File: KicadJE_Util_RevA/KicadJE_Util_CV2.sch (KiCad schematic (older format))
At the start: 53 parts, among them J201 SawOut3, J202 SineOut4, Q201 MMBT3906, Q202 UMX1N, SW201 Octave (3 state), U201 TL072, U202 TL072

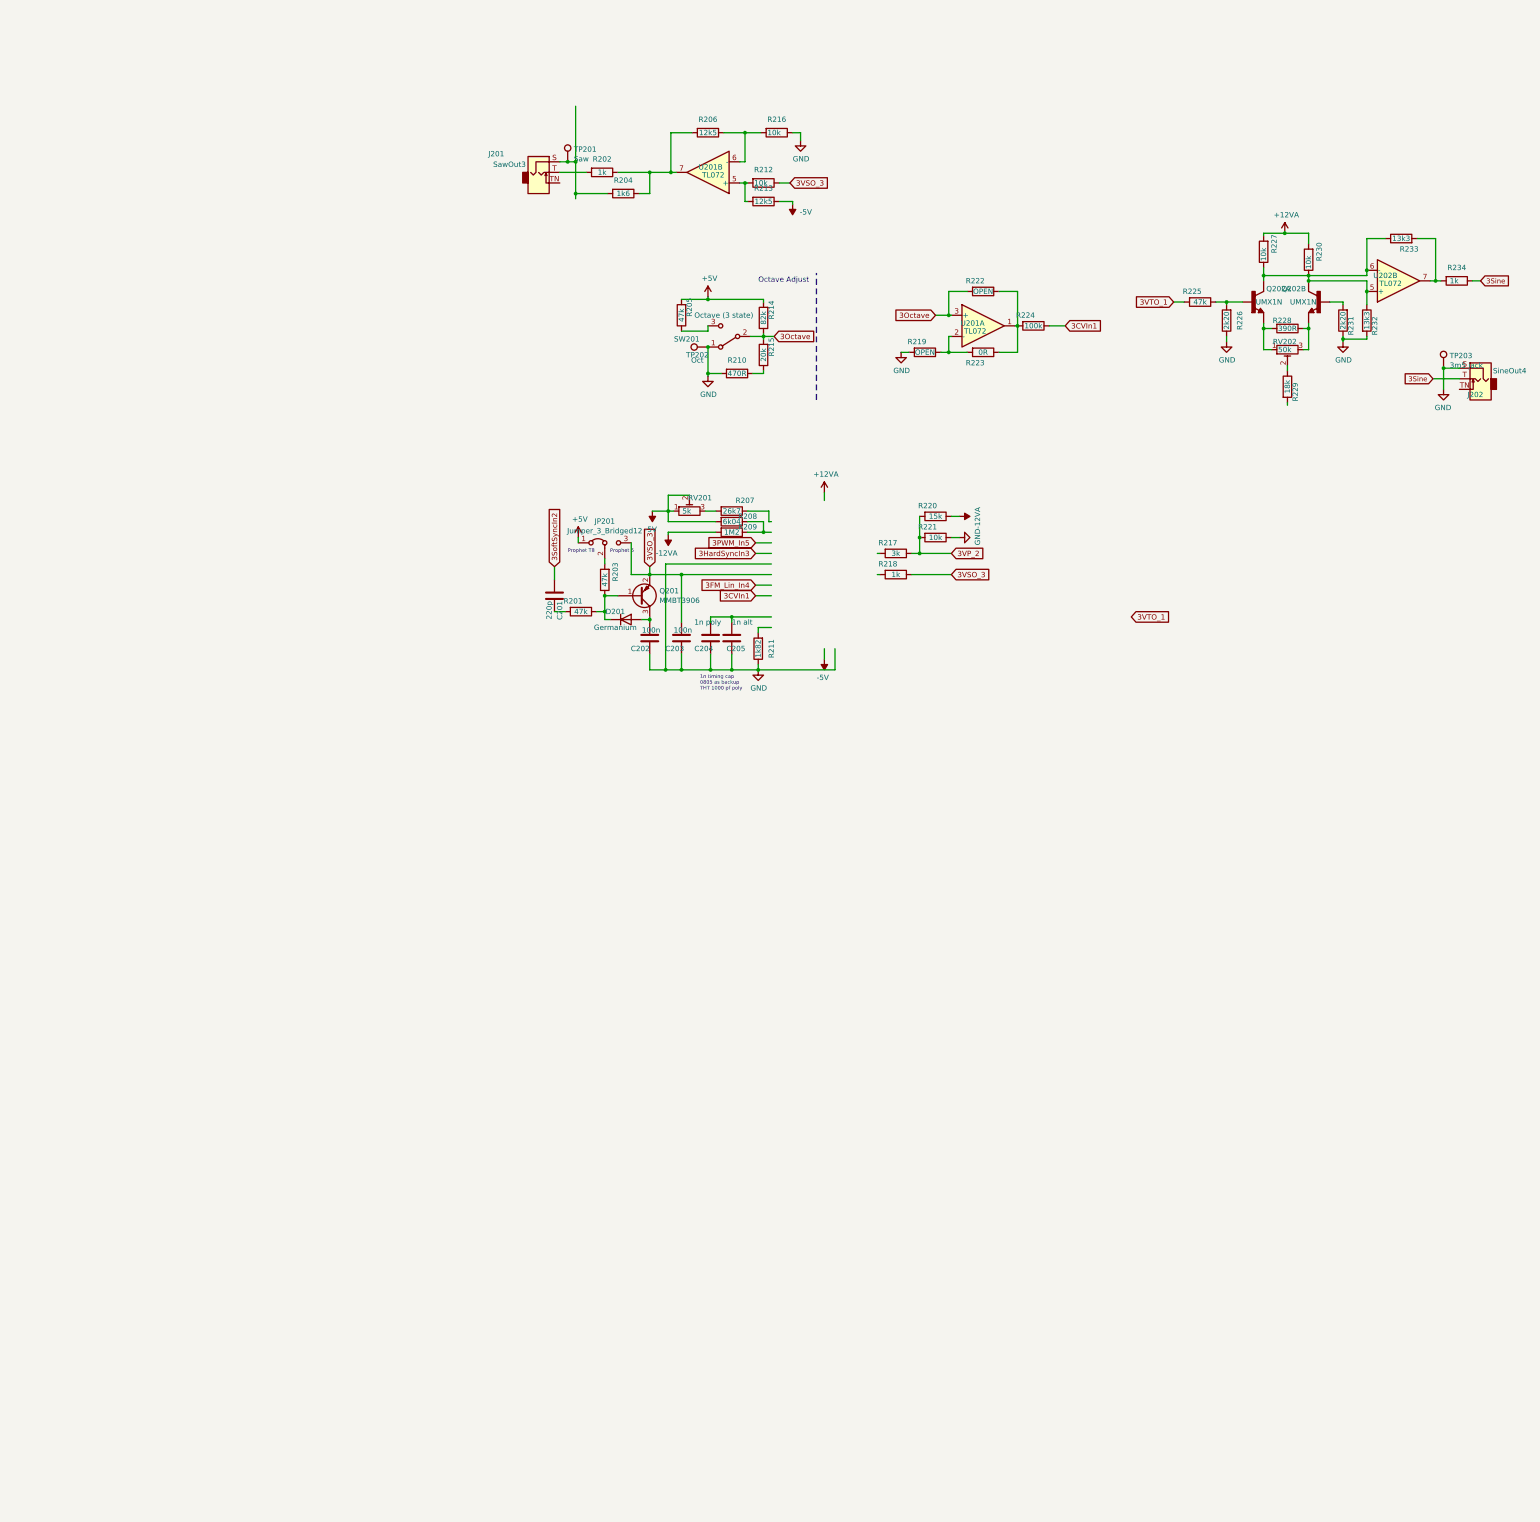
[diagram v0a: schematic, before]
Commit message: fix flow
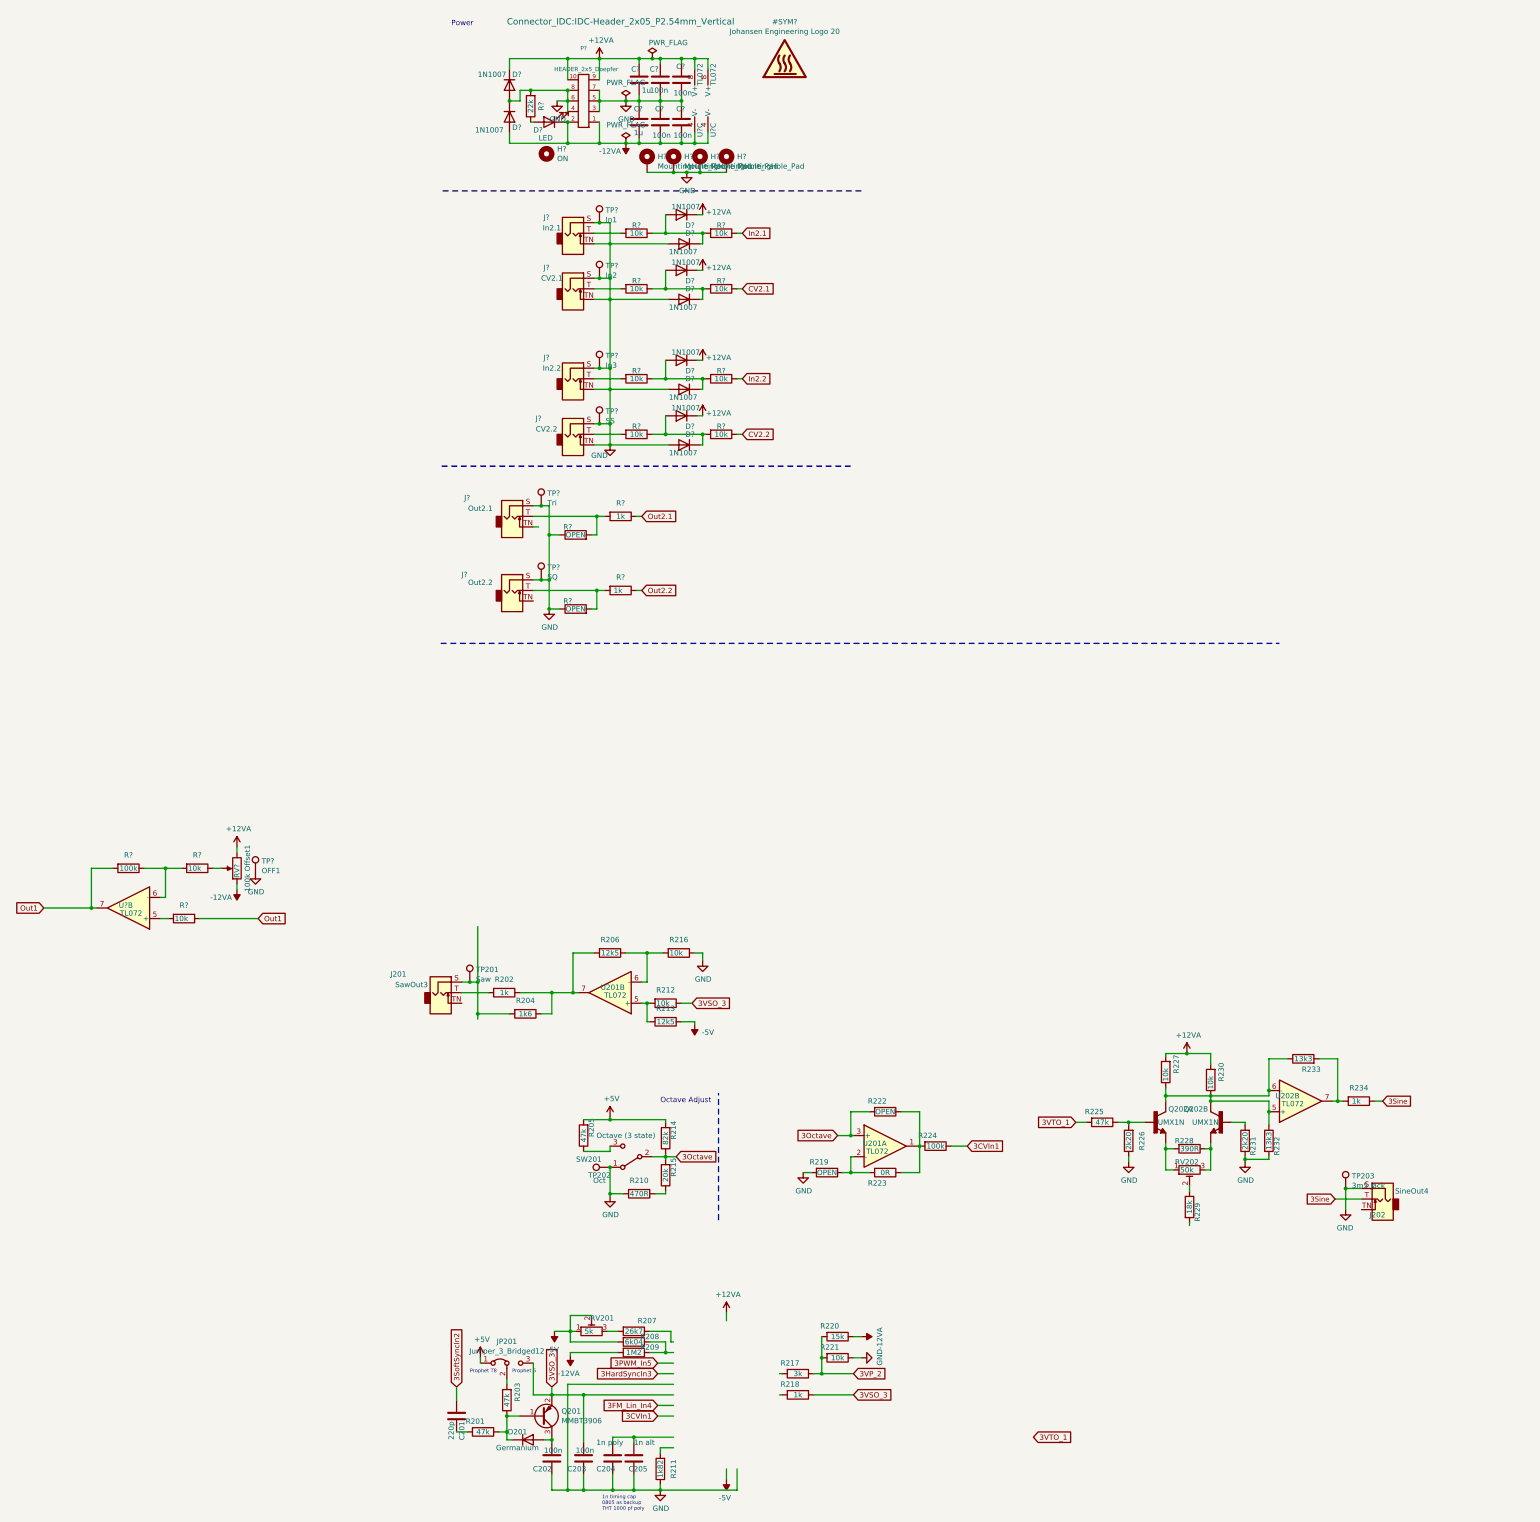
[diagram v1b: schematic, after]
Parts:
- added C? (x2): 1u, Capacitor_SMD:C_1206_3216Metric_Pad1.42x1.75mm_HandSolder, symbol Device:C
- added C? (x4): 100n, Capacitor_SMD:C_0805_2012Metric_Pad1.15x1.40mm_HandSolder, symbol Device:C
- added D? (x10): 1N1007, Diode_SMD:D_SOD-123, symbol Device:D
- added D?: LED, LED_SMD:LED_0805_2012Metric_Pad1.15x1.40mm_HandSolder, symbol Device:LED
- added H? (x4): MountingHole_Pad, AJ:MountingHole_Eurorack3, symbol Mechanical:MountingHole_Pad
- added H?: ON, AJ:LED_Hole_3mm, symbol Mechanical:MountingHole
- added J?: In2.1, AJ-Dropbox-Kicad:PJ301SM, symbol Connector:AudioJack2_SwitchT
- added J?: CV2.1, AJ-Dropbox-Kicad:PJ301SM, symbol Connector:AudioJack2_SwitchT
- added J?: Out2.1, AJ-Dropbox-Kicad:PJ301SM, symbol Connector:AudioJack2_SwitchT
- added J?: CV2.2, AJ-Dropbox-Kicad:PJ301SM, symbol Connector:AudioJack2_SwitchT
- added J?: Out2.2, AJ-Dropbox-Kicad:PJ301SM, symbol Connector:AudioJack2_SwitchT
- added J?: In2.2, AJ-Dropbox-Kicad:PJ301SM, symbol Connector:AudioJack2_SwitchT
- added P?: HEADER_2x5_Doepfer, Connector_IDC:IDC-Header_2x05_P2.54mm_Vertical, symbol Eurorack:HEADER_2x5_Doepfer
- added R? (x10): 10k, Resistor_SMD:R_0805_2012Metric_Pad1.15x1.40mm_HandSolder, symbol Device:R
- added R? (x2): 1k, Resistor_SMD:R_0805_2012Metric_Pad1.15x1.40mm_HandSolder, symbol Device:R
- added R?: 22k, Resistor_SMD:R_0805_2012Metric_Pad1.15x1.40mm_HandSolder, symbol Device:R
- added R? (x2): OPEN, Resistor_SMD:R_0805_2012Metric_Pad1.15x1.40mm_HandSolder, symbol Device:R
- added R?: 100k, Resistor_SMD:R_0805_2012Metric_Pad1.15x1.40mm_HandSolder, symbol Device:R
- added RV?: 100k Offset1, AJ-Dropbox-Kicad:Potentiometer_China_RK09_Single_Vertical_AJ, symbol Envelope-cache-2018-08-04-13-00-04:POT
- added TP?: Tri, AJ:Jack_6m3, symbol Connector:TestPoint
- added TP?: SQ, AJ:Jack_6m3, symbol Connector:TestPoint
- added TP?: SS, AJ:Jack_6m3, symbol Connector:TestPoint
- added TP?: In3, AJ:Jack_6m3, symbol Connector:TestPoint
- added TP?: In2, AJ:Jack_6m3, symbol Connector:TestPoint
- added TP?: In1, AJ:Jack_6m3, symbol Connector:TestPoint
- added TP?: OFF1, AJ:Pot_6m3_scale1, symbol Connector:TestPoint
- added U? (x3): TL072, AJ-Dropbox-Kicad:AJ_SO-8_5.3x6.2mm_P1.27mm, symbol Amplifier_Operational:TL072
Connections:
- net labels added: CV2.1, CV2.2, In2.1, In2.2, Out1, Out2.1, Out2.2
- wire segments 170 -> 319
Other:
- note added: "Power"
- moved on the sheet: C201, C202, C203, C204, C205, D201, J201, J202, JP201, Q201, Q202A, Q202B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

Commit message: Glide initiated
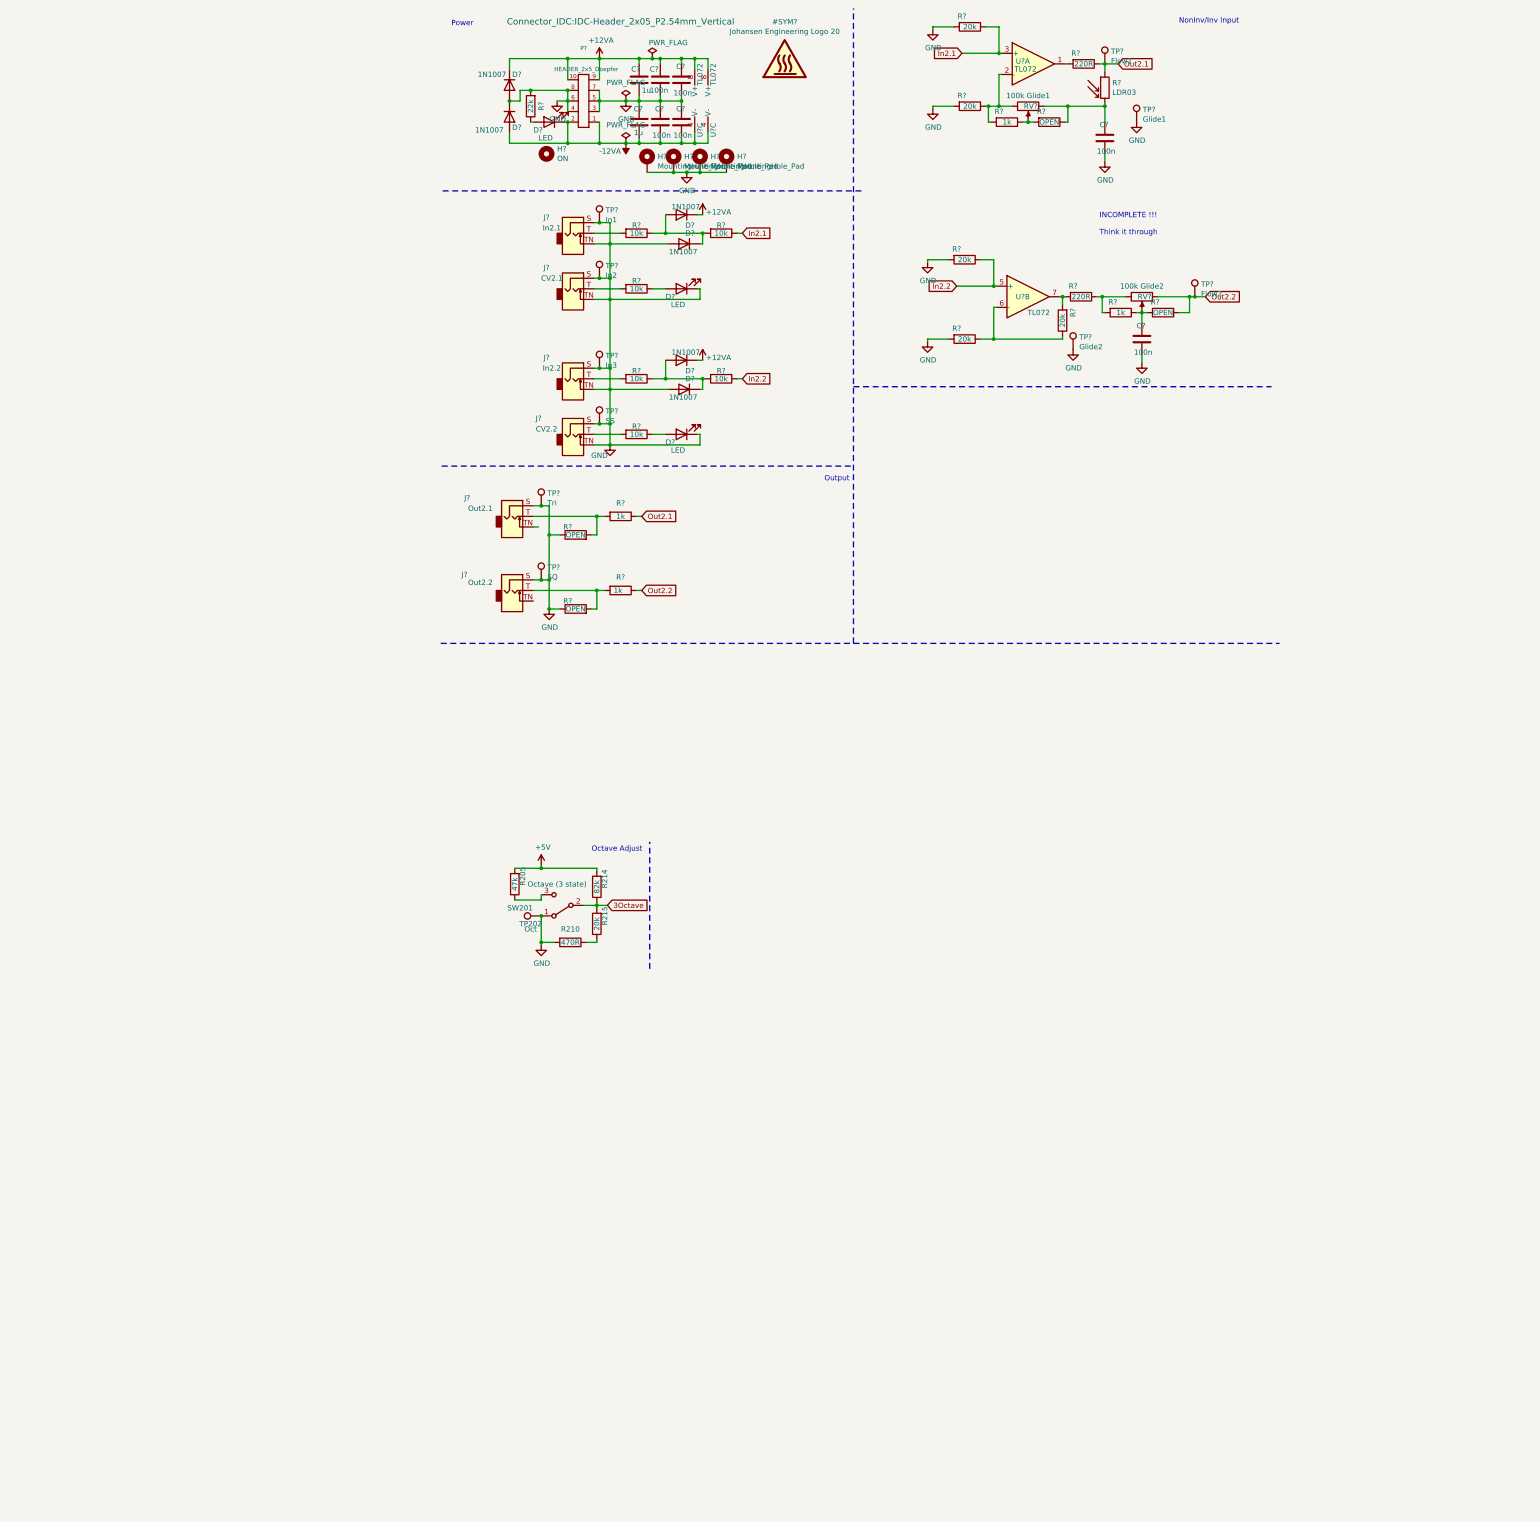
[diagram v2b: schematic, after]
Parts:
- removed C201: 220p, Capacitor_SMD:C_0805_2012Metric_Pad1.15x1.40mm_HandSolder, symbol Device:C
- removed C202, C203: 100n, Capacitor_SMD:C_0805_2012Metric_Pad1.15x1.40mm_HandSolder, symbol Device:C
- removed C204: 1n poly, Capacitor_THT:C_Rect_L7.0mm_W2.0mm_P5.00mm, symbol Device:C
- removed C205: 1n alt, Capacitor_SMD:C_0805_2012Metric_Pad1.15x1.40mm_HandSolder, symbol Device:C
- removed D201: Germanium, Diode_THT:D_A-405_P7.62mm_Horizontal, symbol Device:D
- removed D? (x4): 1N1007, Diode_SMD:D_SOD-123, symbol Device:D
- removed J201: SawOut3, AJ-Dropbox-Kicad:PJ301SM, symbol Connector:AudioJack2_SwitchT
- removed J202: SineOut4, AJ-Dropbox-Kicad:PJ301SM, symbol Connector:AudioJack2_SwitchT
- removed JP201: Jumper_3_Bridged12, Jumper:SolderJumper-3_P1.3mm_Bridged12_Pad1.0x1.5mm_NumberLabels, symbol Jumper:Jumper_3_Bridged12
- removed Q201: MMBT3906, Package_TO_SOT_SMD:SOT-23, symbol Transistor_BJT:MMBT3906
- removed Q202: UMX1N, AJ:UMX1N_UMT6_DualNPN, symbol UMX1N:UMX1N
- removed R201, R203, R225: 47k, Resistor_SMD:R_0805_2012Metric_Pad1.15x1.40mm_HandSolder, symbol Device:R
- removed R202, R218, R234: 1k, Resistor_SMD:R_0805_2012Metric_Pad1.15x1.40mm_HandSolder, symbol Device:R
- removed R204: 1k6, Resistor_SMD:R_0805_2012Metric_Pad1.15x1.40mm_HandSolder, symbol Device:R
- removed R206, R213: 12k5, Resistor_SMD:R_0805_2012Metric_Pad1.15x1.40mm_HandSolder, symbol Device:R
- removed R207: 26k7, Resistor_SMD:R_0805_2012Metric_Pad1.15x1.40mm_HandSolder, symbol Device:R
- removed R208: 6k04, Resistor_SMD:R_0805_2012Metric_Pad1.15x1.40mm_HandSolder, symbol Device:R
- removed R209: 1M2, Resistor_SMD:R_0805_2012Metric_Pad1.15x1.40mm_HandSolder, symbol Device:R
- removed R211: 1k82, Resistor_SMD:R_0805_2012Metric_Pad1.15x1.40mm_HandSolder, symbol Device:R
- removed R212, R216, R221, R227, R230, R? (x5): 10k, Resistor_SMD:R_0805_2012Metric_Pad1.15x1.40mm_HandSolder, symbol Device:R
- removed R217: 3k, Resistor_SMD:R_0805_2012Metric_Pad1.15x1.40mm_HandSolder, symbol Device:R
- removed R219, R222: OPEN, Resistor_SMD:R_0805_2012Metric_Pad1.15x1.40mm_HandSolder, symbol Device:R
- removed R220: 15k, Resistor_SMD:R_0805_2012Metric_Pad1.15x1.40mm_HandSolder, symbol Device:R
- removed R223: 0R, Resistor_SMD:R_0805_2012Metric_Pad1.15x1.40mm_HandSolder, symbol Device:R
- removed R224, R?: 100k, Resistor_SMD:R_0805_2012Metric_Pad1.15x1.40mm_HandSolder, symbol Device:R
- removed R226, R231: 2k20, Resistor_SMD:R_0805_2012Metric_Pad1.15x1.40mm_HandSolder, symbol Device:R
- removed R228: 390R, Resistor_SMD:R_0805_2012Metric_Pad1.15x1.40mm_HandSolder, symbol Device:R
- removed R229: 18k, Resistor_SMD:R_0805_2012Metric_Pad1.15x1.40mm_HandSolder, symbol Device:R
- removed R232, R233: 13k3, Resistor_SMD:R_0805_2012Metric_Pad1.15x1.40mm_HandSolder, symbol Device:R
- removed RV201: 5k, Potentiometer_THT:Potentiometer_Bourns_3296W_Vertical, symbol Device:R_POT_TRIM
- removed RV202: 50k, Potentiometer_THT:Potentiometer_Bourns_3296W_Vertical, symbol Device:R_POT_TRIM
- removed RV?: 100k Offset1, AJ-Dropbox-Kicad:Potentiometer_China_RK09_Single_Vertical_AJ, symbol Envelope-cache-2018-08-04-13-00-04:POT
- removed TP201: Saw, AJ:Jack_6m3, symbol Connector:TestPoint
- removed TP203: 3m5 jack, AJ:Jack_6m3, symbol Connector:TestPoint
- removed TP?: OFF1, AJ:Pot_6m3_scale1, symbol Connector:TestPoint
- removed U201, U202, U?: TL072, AJ-Dropbox-Kicad:AJ_SO-8_5.3x6.2mm_P1.27mm, symbol Amplifier_Operational:TL072
- added C? (x2): 100n, Capacitor_SMD:C_0805_2012Metric_Pad1.15x1.40mm_HandSolder, symbol Device:C
- added D? (x2): LED, LED_THT:LED_D3.0mm, symbol Device:LED
- added R? (x5): 20k, Resistor_SMD:R_0805_2012Metric_Pad1.15x1.40mm_HandSolder, symbol Device:R
- added R? (x2): 220R, Resistor_SMD:R_0805_2012Metric_Pad1.15x1.40mm_HandSolder, symbol Device:R
- added R? (x2): OPEN, Resistor_SMD:R_0805_2012Metric_Pad1.15x1.40mm_HandSolder, symbol Device:R
- added R? (x2): 1k, Resistor_SMD:R_0805_2012Metric_Pad1.15x1.40mm_HandSolder, symbol Device:R
- added R?: 10k, Resistor_SMD:R_0805_2012Metric_Pad1.15x1.40mm_HandSolder, symbol Device:R
- added R?: LDR03, OptoDevice:R_LDR_10x8.5mm_P7.6mm_Vertical, symbol Sensor_Optical:LDR03
- added RV?: 100k Glide1, AJ-Dropbox-Kicad:Potentiometer_China_RK09_Single_Vertical_AJ, symbol Envelope-cache-2018-08-04-13-00-04:POT
- added RV?: 100k Glide2, AJ-Dropbox-Kicad:Potentiometer_China_RK09_Single_Vertical_AJ, symbol Envelope-cache-2018-08-04-13-00-04:POT
- added TP?: Glide2, AJ:Pot_6m3_scale1, symbol Connector:TestPoint
- added TP?: Glide1, AJ:Pot_6m3_scale1, symbol Connector:TestPoint
- added TP?: Flow1, TestPoint:TestPoint_THTPad_2.0x2.0mm_Drill1.0mm, symbol Connector:TestPoint
- added TP?: Flow2, TestPoint:TestPoint_THTPad_2.0x2.0mm_Drill1.0mm, symbol Connector:TestPoint
- added U? (x2): TL072, AJ-Dropbox-Kicad:AJ_SO-8_5.3x6.2mm_P1.27mm, symbol Amplifier_Operational:TL072
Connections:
- net labels removed: -5V, 3CVIn1, 3FM_Lin_In4, 3HardSyncIn3, 3PWM_In5, 3Sine, 3SoftSyncIn2, 3VP_2, 3VSO_3, 3VTO_1, CV2.1, CV2.2, Out1
- wire segments 319 -> 198
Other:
- note added: "INCOMPLETE !!!\n\nThink it through"
- note added: "NonInv/Inv Input"
- note added: "Output"
- note removed: "1n timing cap\n0805 as backup\nTHT 1000 pf poly"
- note removed: "Prophet 5"
- note removed: "Prophet T8"
- moved on the sheet: R205, R210, R214, R215, SW201, TP202
